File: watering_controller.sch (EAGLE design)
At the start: 12 parts, among them IC2 7805T, J1 DCJ0202, J2 DCJ0202, Q1 IRLZ44Z

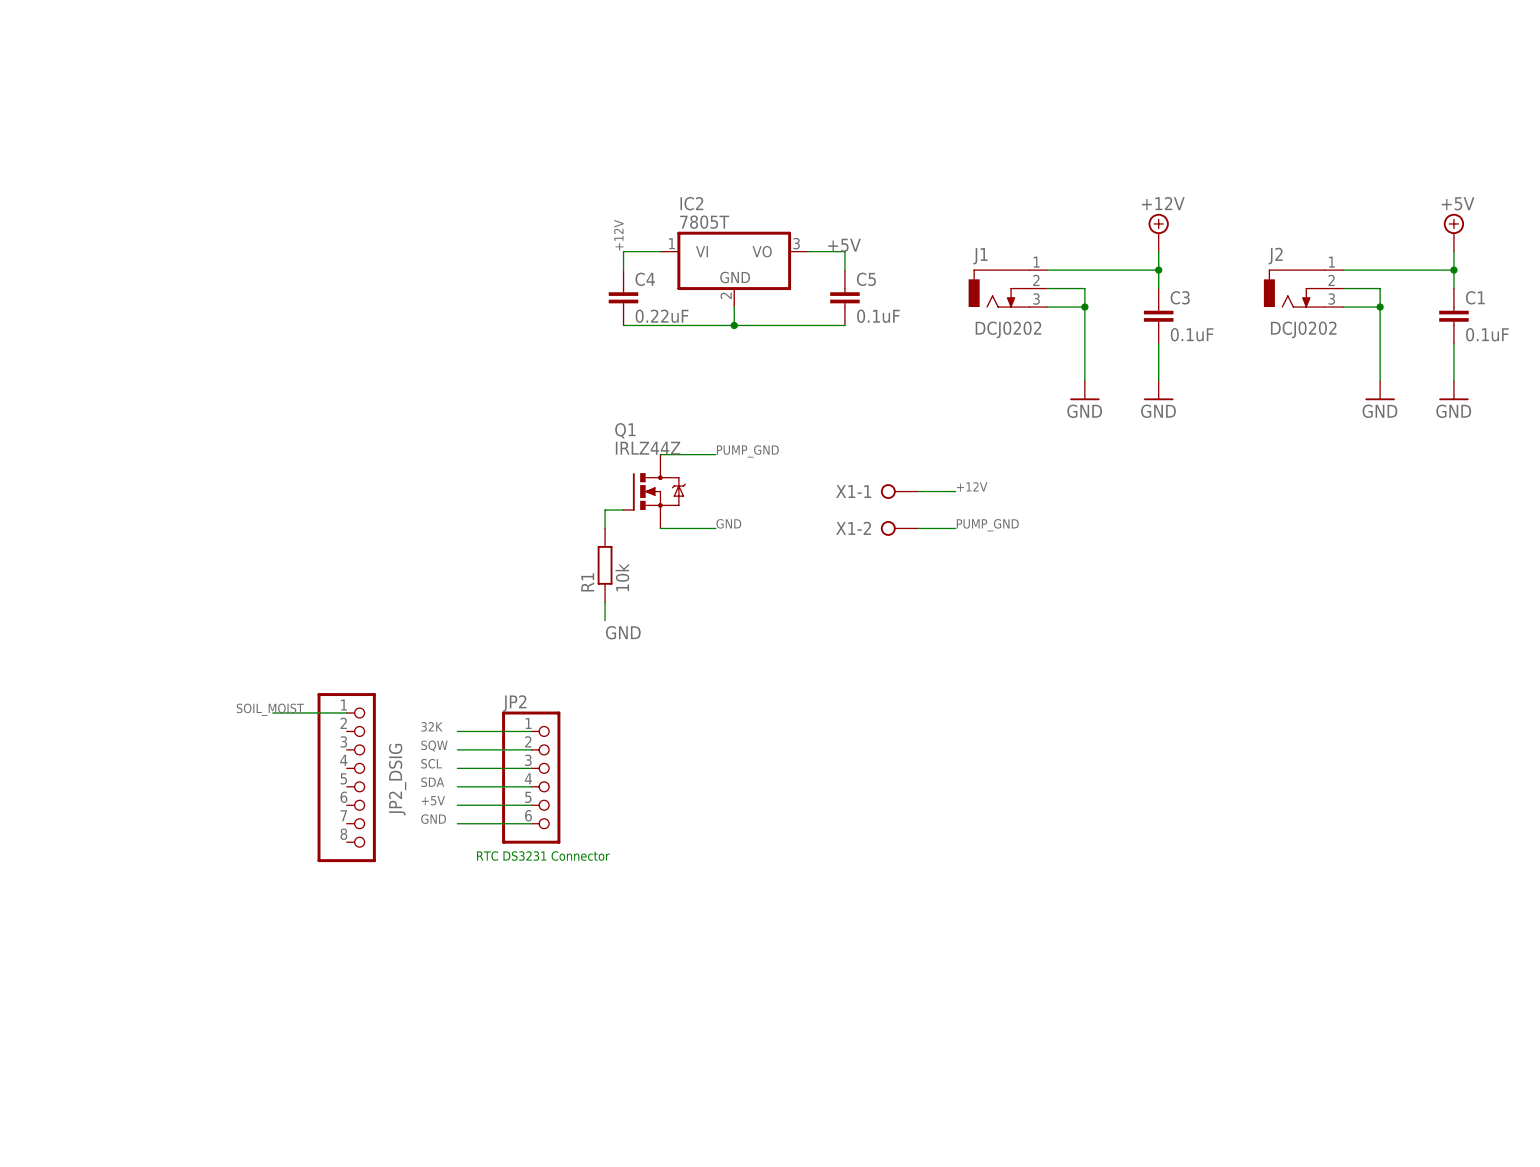
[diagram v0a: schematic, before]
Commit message: Update smd version
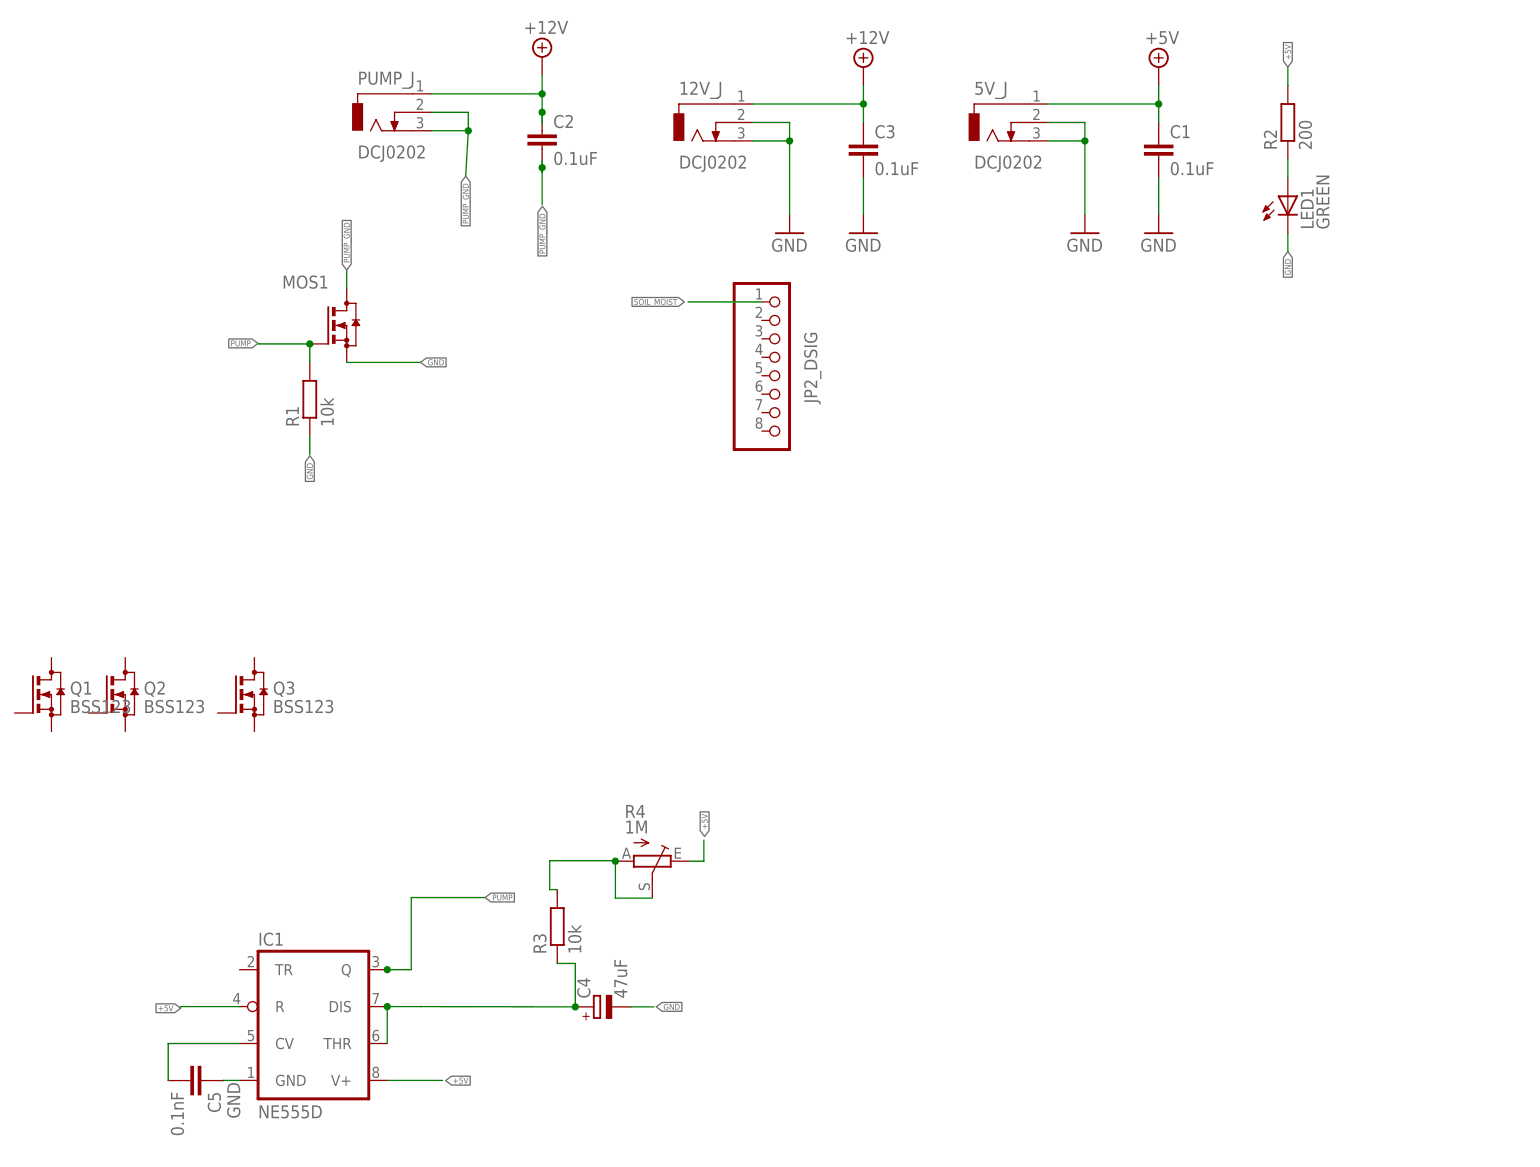
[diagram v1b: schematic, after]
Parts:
- removed IC2: 7805T, linear:7805T
- removed J1, J2: DCJ0202, con-jack:DCJ0202
- removed JP2: (no value), pinhead:PINHD-1X6
- removed X1: (no value), con-wago-508:W237-02P
- added 12V_J, 5V_J, PUMP_J: DCJ0202, con-jack:DCJ0202
- added C2: 0.1uF, rcl:C-EUC0805
- added IC1: NE555D, linear:NE555D
- added LED1: GREEN, led:LEDSML0805
- added MOS1: (no value), ckr_parts:FDN359BN
- added Q2, Q3: BSS123, transistor-small-signal:BSS123
- added R2: 200, resistor:R-EU_M0805
- added R3: 10k, resistor:R-EU_M0805
- added R4: 1M, pot:TRIM_EU-B25P
- C1, C3: device rcl:C-EU025-025X050 -> rcl:C-EUC0805
- C4: value 0.22uF -> 47uF; device rcl:C-EU025-025X050 -> rcl:CPOL-EUA/3216-18R
- C5: value 0.1uF -> 0.1nF; device rcl:C-EU025-025X050 -> rcl:C-EUC0805
- Q1: value IRLZ44Z -> BSS123; device transistor-power:IRLZ44Z -> transistor-small-signal:BSS123
- R1: device resistor:R-EU_0204/5 -> resistor:R-EU_M0805
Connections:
- removed net +12V: C4.1, IC2.VI, X1-1.KL
- removed net 32K: JP2.1
- removed net GND1: C4.2, C5.2, IC2.GND
- removed net SCL: JP2.3
- removed net SDA: JP2.4
- removed net SQW: JP2.2
- new net N$2: R3.2, R4.A, R4.S
- new net N$3: C4.+, IC1.DIS, IC1.THR, R3.1
- new net N$4: LED1.A, R2.1
- new net PUMP: IC1.Q, MOS1.G, R1.2
- net +5V: now also IC1.R, IC1.V+, R2.2, R4.E; no longer C5.1, IC2.VO, JP2.5
- net +9V: now also 12V_J.1, 5V_J.1, C2.1, PUMP_J.1; no longer J1.1, J2.1
- net GND: now also 12V_J.2, 12V_J.3, 5V_J.2, 5V_J.3, C4.-, C5.1, IC1.GND, LED1.C, MOS1.S; no longer J1.2, J1.3, J2.2, J2.3, JP2.6, Q1.S
- net N$1: now also C5.2, IC1.CV; no longer Q1.G, R1.2
- net PUMP_GND: now also C2.2, MOS1.D, PUMP_J.2, PUMP_J.3; no longer Q1.D, X1-2.KL
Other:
- note removed: "RTC DS3231 Connector"
- moved on the sheet: C1, C3, C5, R1
